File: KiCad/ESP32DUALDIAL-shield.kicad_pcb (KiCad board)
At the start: 2 copper layers, 160 x 70 mm, 7 parts

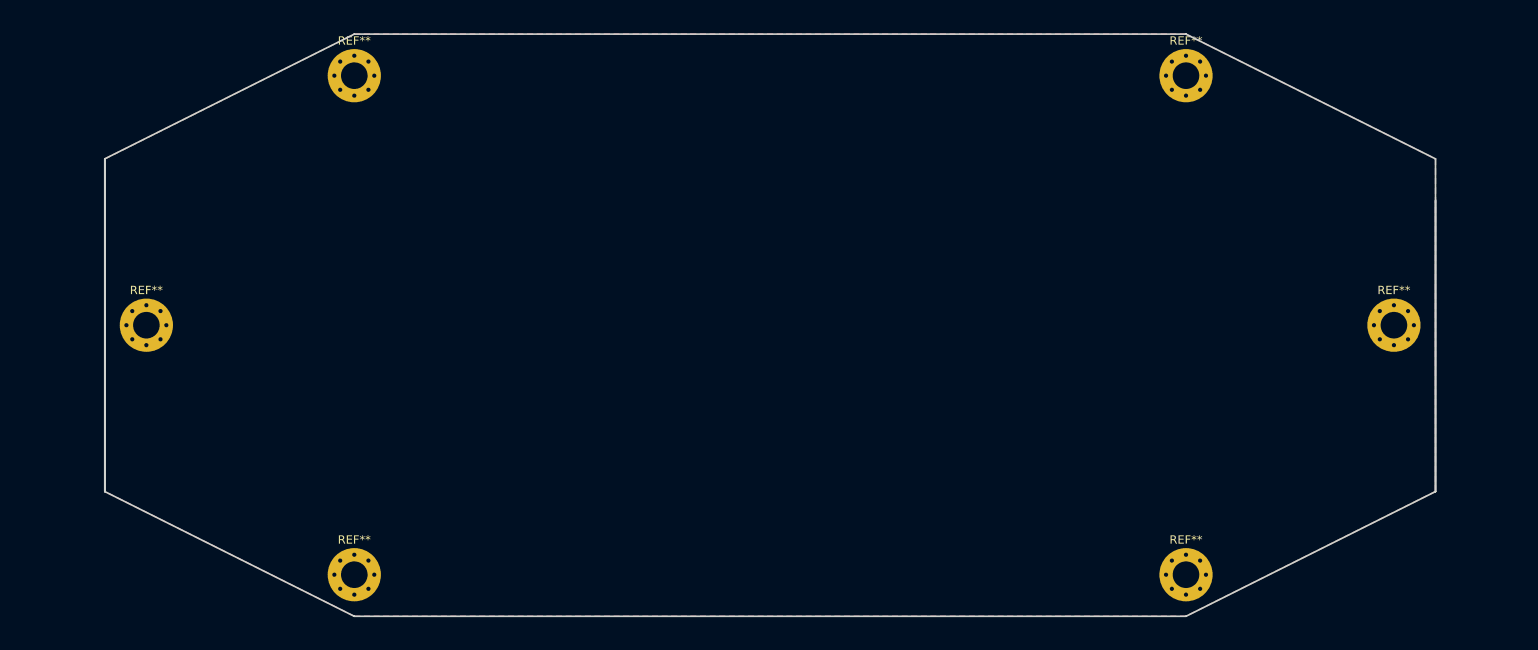
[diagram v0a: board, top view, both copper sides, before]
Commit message: version 20210119
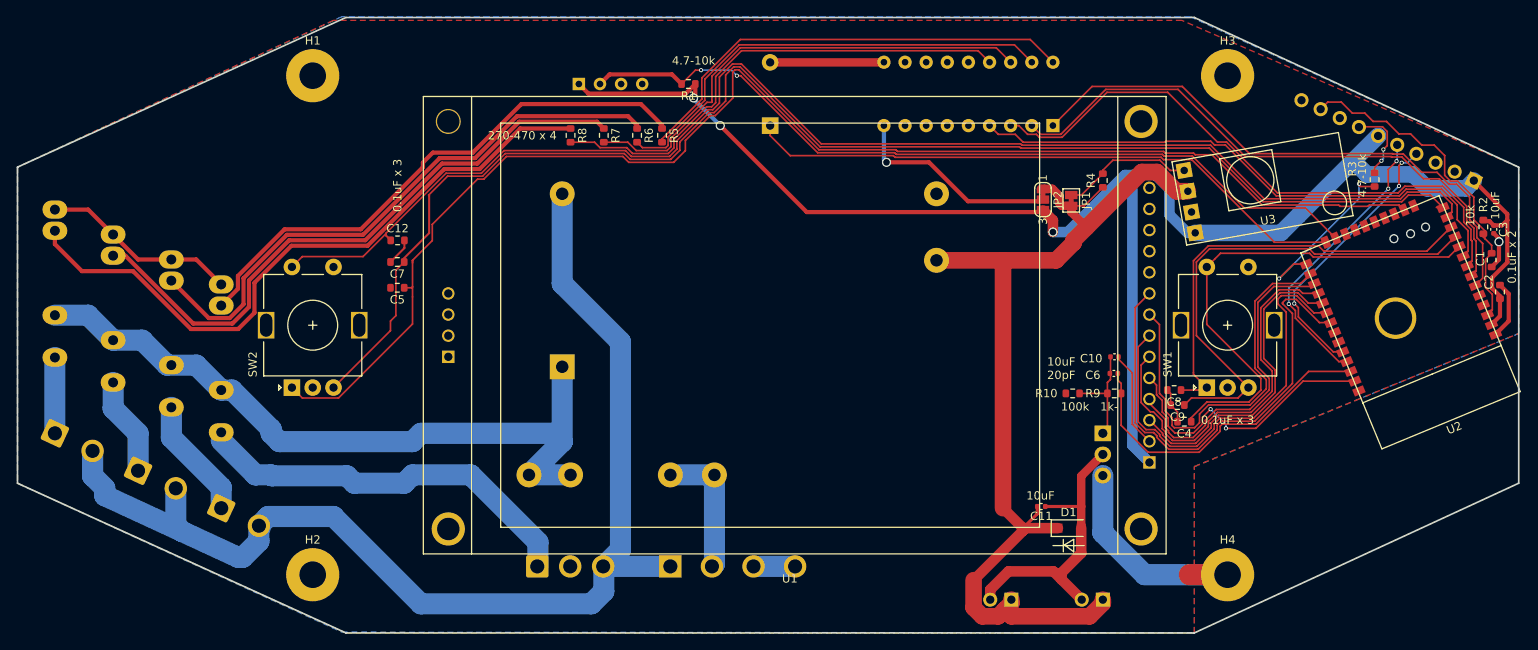
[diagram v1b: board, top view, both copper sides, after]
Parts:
- removed the REF** at (165.0, 80.0)
- removed the REF** at (190.0, 110.0)
- removed the REF** at (40.0, 110.0)
- removed the REF** at (65.0, 80.0)
- removed the REF** at (165.0, 140.0)
- removed the REF** at (65.0, 140.0)
- added BZ1: Buzzer, Buzzer_Beeper:Buzzer_12x9.5RM7.6, B.Cu at (115.0, 86.0)
- added C1: 0.1uF, Resistor_SMD:R_0603_1608Metric, F.Cu at (201.8, 102.2)
- added C10: 10u, Capacitor_SMD:C_0402_1005Metric, F.Cu at (156.4, 113.8)
- added C11: 10u, Capacitor_SMD:C_0402_1005Metric, F.Cu at (147.6, 131.8)
- added C12: 0.1uF, Resistor_SMD:R_0603_1608Metric, F.Cu at (70.2, 99.8)
- added C2: 0.1uF, Resistor_SMD:R_0603_1608Metric, F.Cu at (202.8, 106.0)
- added C3: 10u, Capacitor_SMD:C_0402_1005Metric, F.Cu at (202.0, 98.5)
- added C4: 0.1uF, Resistor_SMD:R_0603_1608Metric, F.Cu at (164.8, 121.6)
- added C5: 0.1uF, Resistor_SMD:R_0603_1608Metric, F.Cu at (70.2, 105.5)
- added C6: 20p, Capacitor_SMD:C_0402_1005Metric, F.Cu at (156.3, 115.8)
- added C7: 0.1uF, Resistor_SMD:R_0603_1608Metric, F.Cu at (70.2, 102.4)
- added C8: 0.1uF, Resistor_SMD:R_0603_1608Metric, F.Cu at (163.6, 117.8)
- added C9: 0.1uF, Resistor_SMD:R_0603_1608Metric, F.Cu at (164.0, 119.6)
- added D1: D_Schottky, Diode_SMD:D_SOD-123F, F.Cu at (151.0, 134.4)
- added F1: Fuse, library:20mmFuse_P5x2, B.Cu at (97.0, 128.0)
- added H1: MountingHole_Pad, MountingHole:MountingHole_3.2mm_M3_Pad, F.Cu at (60.0, 80.0)
- added H2: MountingHole_Pad, MountingHole:MountingHole_3.2mm_M3_Pad, F.Cu at (60.0, 140.0)
- added H3: MountingHole_Pad, MountingHole:MountingHole_3.2mm_M3_Pad, F.Cu at (170.0, 80.0)
- added H4: MountingHole_Pad, MountingHole:MountingHole_3.2mm_M3_Pad, F.Cu at (170.0, 140.0)
- added J1: SERVICE, Connector_PinHeader_2.54mm:PinHeader_1x10_P2.54mm_Vertical, B.Cu at (199.6, 92.6)
- added J2: Conn_01x04_Male, Connector_JST:JST_NV_B04P-NV_1x04_P5.00mm_Vertical, B.Cu at (103.0, 139.0)
- added J3: FAN, Connector_PinSocket_2.54mm:PinSocket_1x02_P2.54mm_Vertical, B.Cu at (144.0, 143.0)
- added J4: FAN, Connector_PinSocket_2.54mm:PinSocket_1x02_P2.54mm_Vertical, B.Cu at (155.0, 143.0)
- added J5: Conn_01x03_Male, Connector_JST:JST_VH_B3P-VH_1x03_P3.96mm_Vertical, B.Cu at (87.0, 139.0)
- added J6: Conn_01x02_Male, Connector_JST:JST_NV_B02P-NV_1x02_P5.00mm_Vertical, B.Cu at (49.0, 132.0)
- added J7: Conn_01x02_Male, Connector_JST:JST_NV_B02P-NV_1x02_P5.00mm_Vertical, B.Cu at (39.0, 127.5)
- added J8: Conn_01x02_Male, Connector_JST:JST_NV_B02P-NV_1x02_P5.00mm_Vertical, B.Cu at (29.0, 123.0)
- added JP1: Jumper, Jumper:SolderJumper-2_P1.3mm_Bridged_Pad1.0x1.5mm, F.Cu at (151.2, 95.0)
- added JP2: Jumper_NC_Dual, Jumper:SolderJumper-3_P1.3mm_Bridged12_RoundedPad1.0x1.5mm_NumberLabels, F.Cu at (147.8, 94.9)
- added PS1: IRM-20-12, Converter_ACDC:Converter_ACDC_MeanWell_IRM-20-xx_THT, B.Cu at (90.0, 115.0)
- added Q1: Q_NMOS_GDS, Package_TO_SOT_THT:TO-220-3_Vertical, B.Cu at (155.0, 123.0)
- added R1: 103, Resistor_SMD:R_0603_1608Metric, F.Cu at (105.2, 81.0)
- added R10: 100k, Resistor_SMD:R_0603_1608Metric, F.Cu at (151.4, 118.2)
- added R2: 10k, Resistor_SMD:R_0603_1608Metric, F.Cu at (200.8, 98.2)
- added R3: 4.7k, Resistor_SMD:R_0603_1608Metric, F.Cu at (187.7, 92.5)
- added R4: NC, Resistor_SMD:R_0603_1608Metric, F.Cu at (155.0, 92.6)
- added R5: 330, Resistor_SMD:R_0603_1608Metric, F.Cu at (102.0, 87.2)
- added R6: 330, Resistor_SMD:R_0603_1608Metric, F.Cu at (99.0, 87.2)
- added R7: 330, Resistor_SMD:R_0603_1608Metric, F.Cu at (95.0, 87.2)
- added R8: 330, Resistor_SMD:R_0603_1608Metric, F.Cu at (91.0, 87.2)
- added R9: 1k, Resistor_SMD:R_0603_1608Metric, F.Cu at (156.4, 118.2)
- added SW1: Rotary_Encoder_Switch, Rotary_Encoder:RotaryEncoder_Alps_EC11E-Switch_Vertical_H20mm, F.Cu at (167.5, 117.5)
- added SW2: Rotary_Encoder_Switch, Rotary_Encoder:RotaryEncoder_Alps_EC11E-Switch_Vertical_H20mm, F.Cu at (57.5, 117.5)
- added U1: CR2013-MI2120, library:TFT3.2_ILI9341, F.Cu at (115.0, 110.0)
- added U2: ESP-WROOM-32, library:ESP-WROOM-32, F.Cu at (194.0, 114.5)
- added U3: QS-1205CME-3A_MINIDC-DC_12-24Vto5V3A_1.8V_2.5V_3.3V_5V_9V_1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, library:QS-1205CME-3A_MINIDC-DC_12-24Vto5V3A_1.8V_2.5V_3.3V_5V_9V_12V, F.Cu at (174.2, 93.6)
- added U4: DHT11, Sensor:Aosong_DHT11_5.5x12.0_P2.54mm, B.Cu at (92.0, 81.0)
- added U5: S108T02, library:SSR_SHARP_S108T02, B.Cu at (49.0, 114.0)
- added U6: S108T02, library:SSR_SHARP_S108T02, B.Cu at (43.0, 111.0)
- added U7: S108T02, library:SSR_SHARP_S108T02, B.Cu at (36.0, 108.0)
- added U8: S108T02, library:SSR_SHARP_S108T02, B.Cu at (29.0, 105.0)
- added U9: TBD62783A, Package_DIP:DIP-18_W7.62mm, B.Cu at (149.0, 86.0)
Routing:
- net +3V3: track 0.00 -> 195.0 mm, vias 0 -> 3
- net Net-(C5-Pad1): track 0.00 -> 167.8 mm
- net Net-(C7-Pad1): track 0.00 -> 167.7 mm
- net Net-(C12-Pad1): track 0.00 -> 163.5 mm
- net Net-(J2-Pad1): track 0.00 -> 141.3 mm
- net +12V: track 0.00 -> 120.6 mm
- net Net-(R1-Pad2): track 0.00 -> 98.5 mm, vias 0 -> 2
- net GND: track 0.00 -> 97.0 mm, vias 0 -> 4
- net Net-(F1-Pad1): track 0.00 -> 88.1 mm
- net Net-(R8-Pad1): track 0.00 -> 79.9 mm
- net Net-(R7-Pad1): track 0.00 -> 74.6 mm
- net Net-(BZ1-Pad1): track 0.00 -> 73.3 mm
- net OZON1: track 0.00 -> 71.4 mm
- net Net-(R6-Pad1): track 0.00 -> 70.6 mm
- net OZON0: track 0.00 -> 69.9 mm
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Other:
- board size 160 x 70 mm -> 180.5 x 74 mm
- net class 220V added: clearance 1.5, trace_width 2, via_dia 1.5, via_drill 1
- net class 220VSub added: clearance 0.15, trace_width 0.25, via_dia 0.5, via_drill 0.3
- rule pad_to_mask_clearance: 0.2 -> 0
- board text added: "0.1uF x 2"
- board text added: "0.1uF x 3"
- board text added: "100k 1k-"
- board text added: "10k"
- board text added: "10uF"
- board text added: "10uF 20pF"
- board text added: "270-470 x 4"
- board text added: "3V3 GND KEY RXD TXD 3V3 PRG GND RST GND"
- board text added: "4.7-10k"
- board text added: "ACTIVE SCREEN AREA (AA) = 65 x 49mm"
- board text added: "ANTENNA WINDOW"
- board text added: "DIAL ( if 30mm Φ )"
- board text added: "ESP32 ANTENNA"
- board text added: "G D S NMOS"
